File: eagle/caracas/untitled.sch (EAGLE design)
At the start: 8 parts, among them IC1 4027N

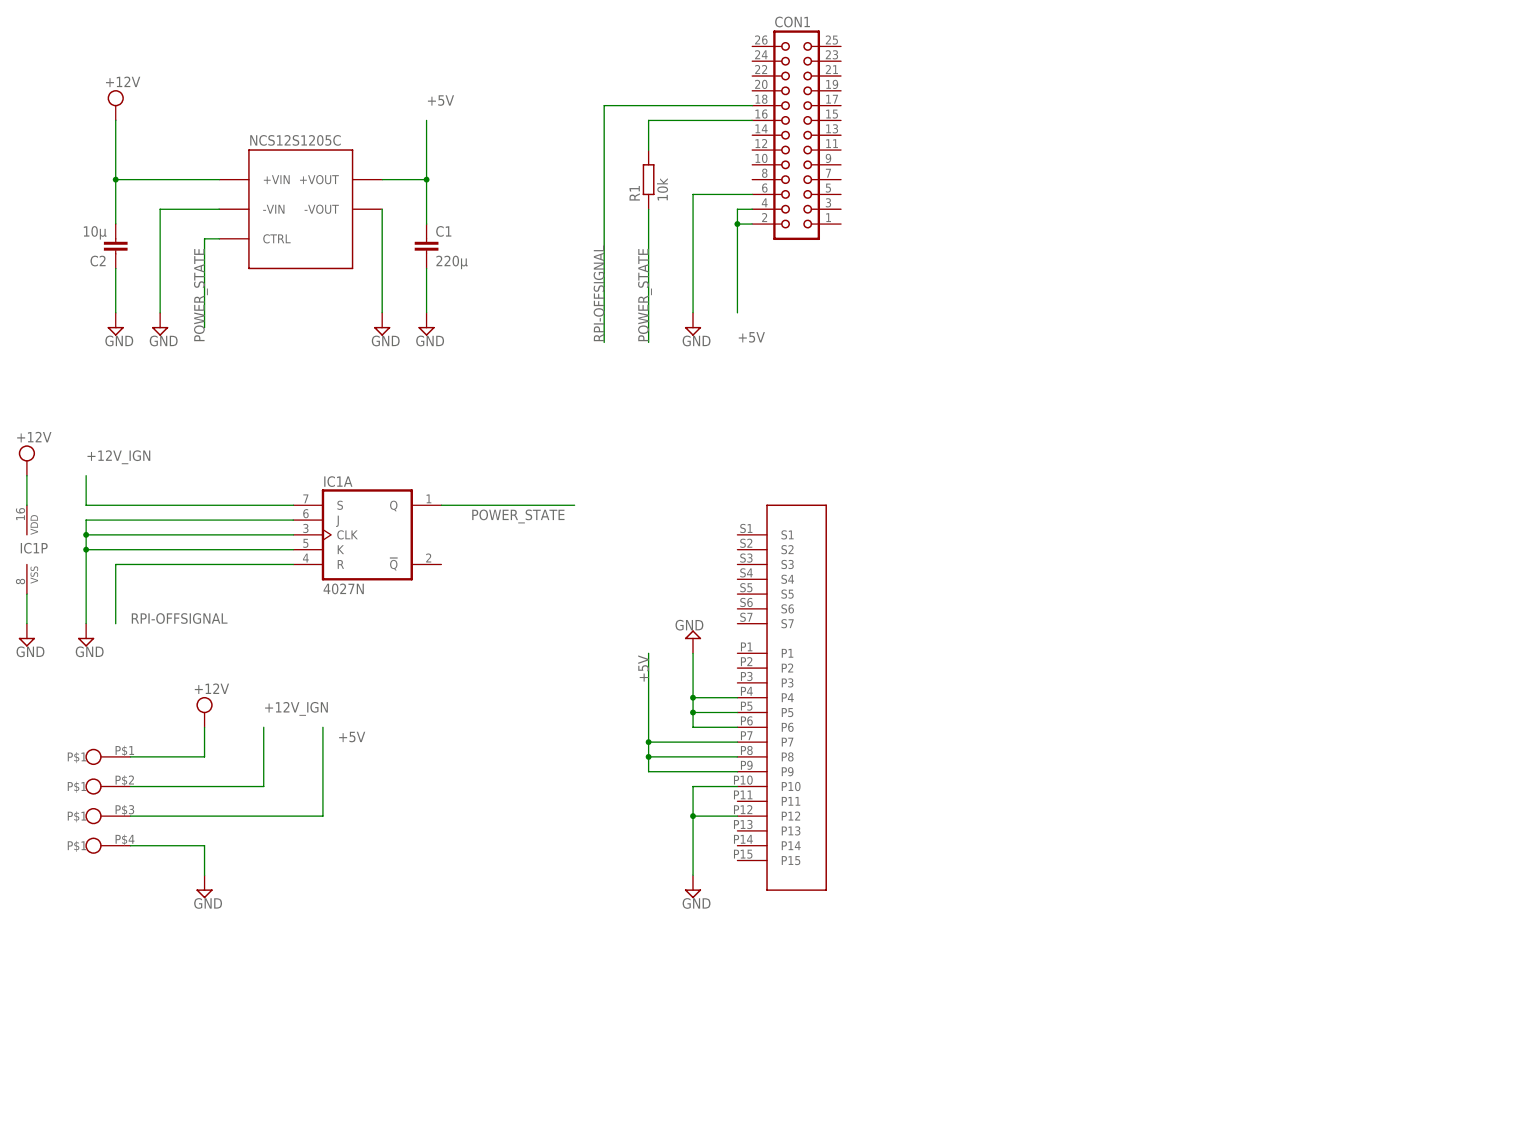
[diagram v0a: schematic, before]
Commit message: Save the board again.
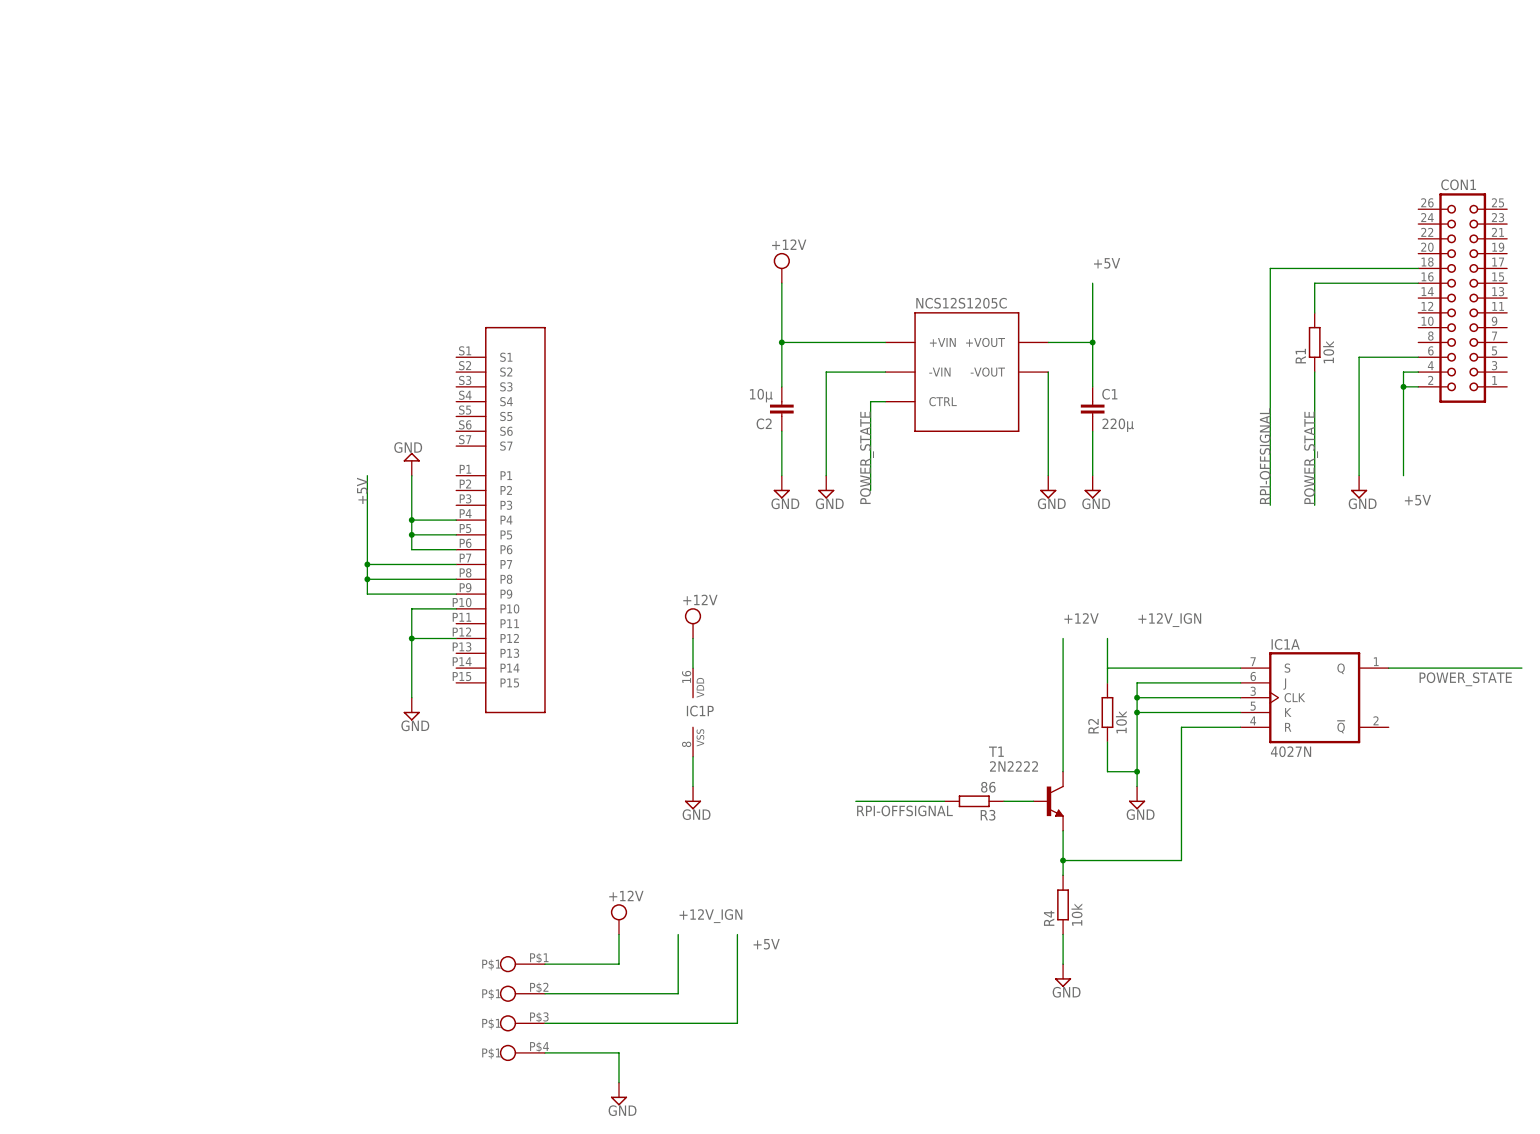
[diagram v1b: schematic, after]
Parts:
- added R2, R4: 10k, rcl:R-EU_0207/10
- added R3: 86, rcl:R-EU_0207/10
- added T1: 2N2222, transistor:2N2222
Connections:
- new net +12V: T1.C
- new net N$1: IC1A.S
- new net N$2: R3.1, T1.B
- new net N$4: IC1A.R, R4.2, T1.E
- net +12V_IGN: now also R2.2; no longer IC1A.S
- net GND: now also R2.1, R4.1
- net RPI-OFFSIGNAL: now also R3.2; no longer IC1A.R
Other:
- moved on the sheet: C1, C2, CON1, IC1A, IC1P, R1

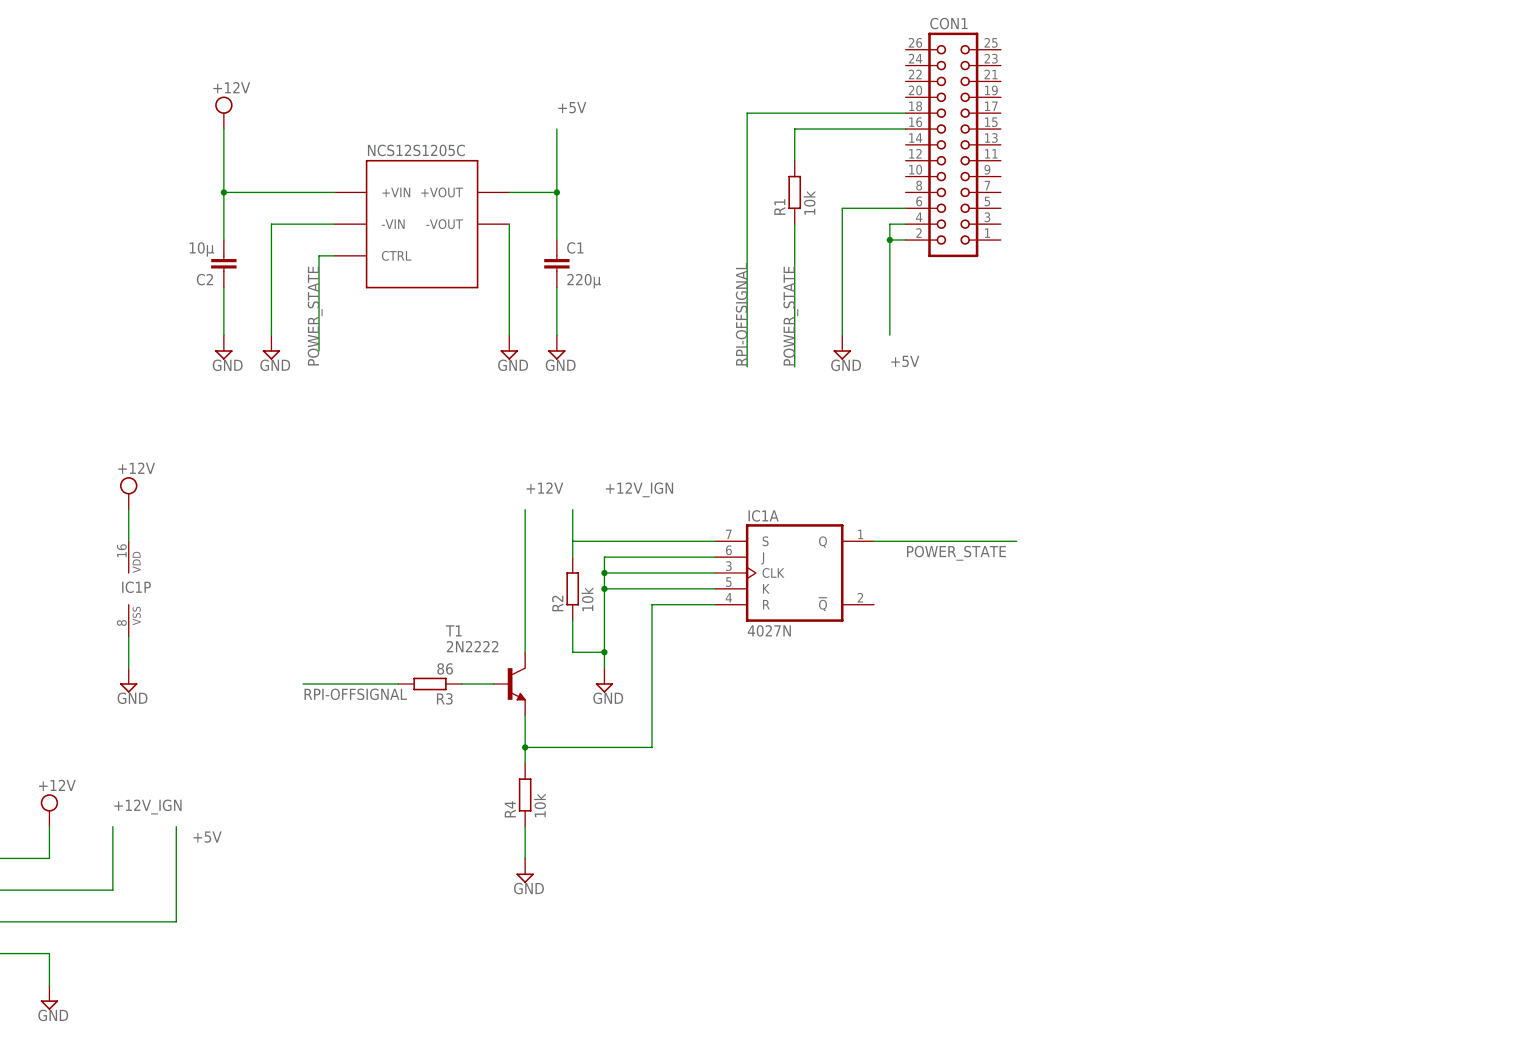
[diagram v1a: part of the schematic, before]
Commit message: WIP on electronics schematics.
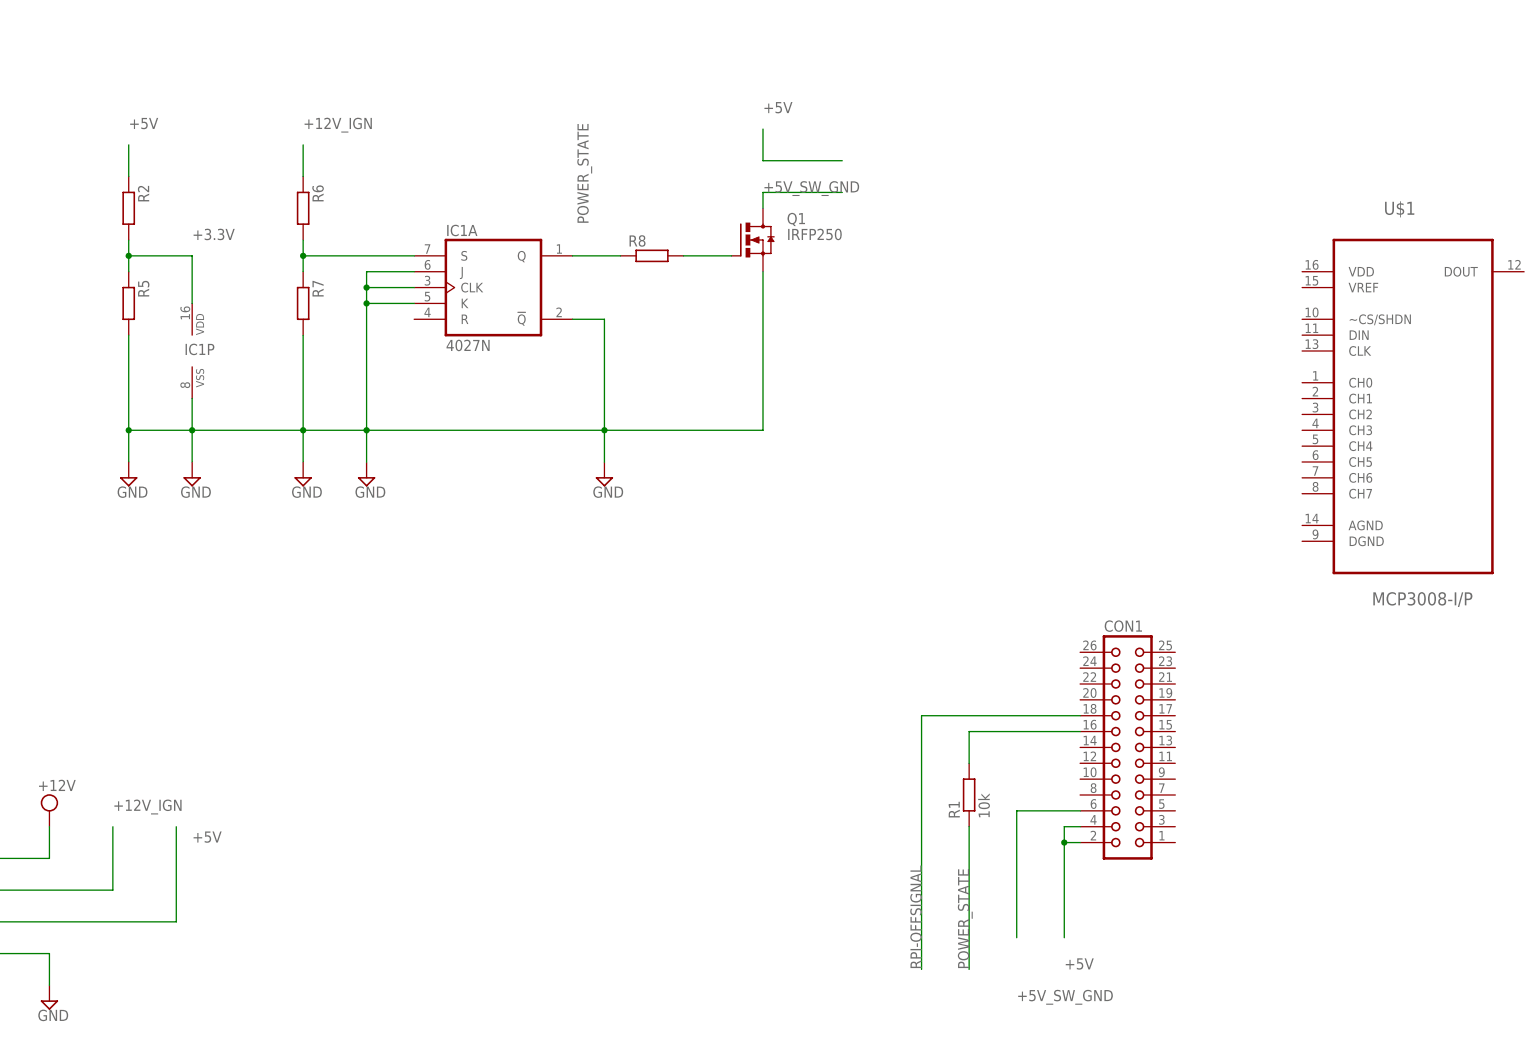
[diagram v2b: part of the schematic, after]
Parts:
- removed C1: 220µ, rcl:C-EU025-024X044
- removed C2: 10µ, rcl:C-EU025-024X044
- removed R3: 86, rcl:R-EU_0207/10
- removed R4: 10k, rcl:R-EU_0207/10
- removed T1: 2N2222, transistor:2N2222
- added Q1: IRFP250, transistor-power:IRFP250
- added R5, R6, R7, R8: (no value), rcl:R-EU_0207/10
- R2: value 10k -> (none)
- U$1: value NCS12S1205C -> MCP3008-I/P; device caracas:NCS12S1205C -> mpc3008:MCP3008-I/P
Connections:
- removed net +12V: T1.C
- removed net N$4: IC1A.R, R4.2, T1.E
- new net +3.3V: IC1P.VDD, R2.2, R5.1
- new net +3.3V1: IC1A.S, R6.2, R7.1
- new net +5V_SW_GND: CON1.6, Q1.D
- net +12V_IGN: now also R6.1; no longer R2.2
- net +5V: now also R2.1; no longer C1.1, U$1.+VOUT
- net GND: now also Q1.S, R5.2, R7.2; no longer C1.2, C2.1, CON1.6, R2.1, R4.1, U$1.-VIN, U$1.-VOUT
- net N$1: now also Q1.G, R8.2; no longer IC1A.S
- net N$2: now also IC1A.!Q; no longer R3.1, T1.B
- net POWER_STATE: now also R8.1; no longer U$1.CTRL
- net RPI-OFFSIGNAL: no longer R3.2
- net VCC: no longer C2.2, IC1P.VDD, U$1.+VIN
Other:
- moved on the sheet: CON1, IC1A, IC1P, R1, R2
